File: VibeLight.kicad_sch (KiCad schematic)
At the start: 7 parts, among them SW1 SW_Push, SW2 SW_Push, U1 OPT3002-ALS, U2 ADXL343

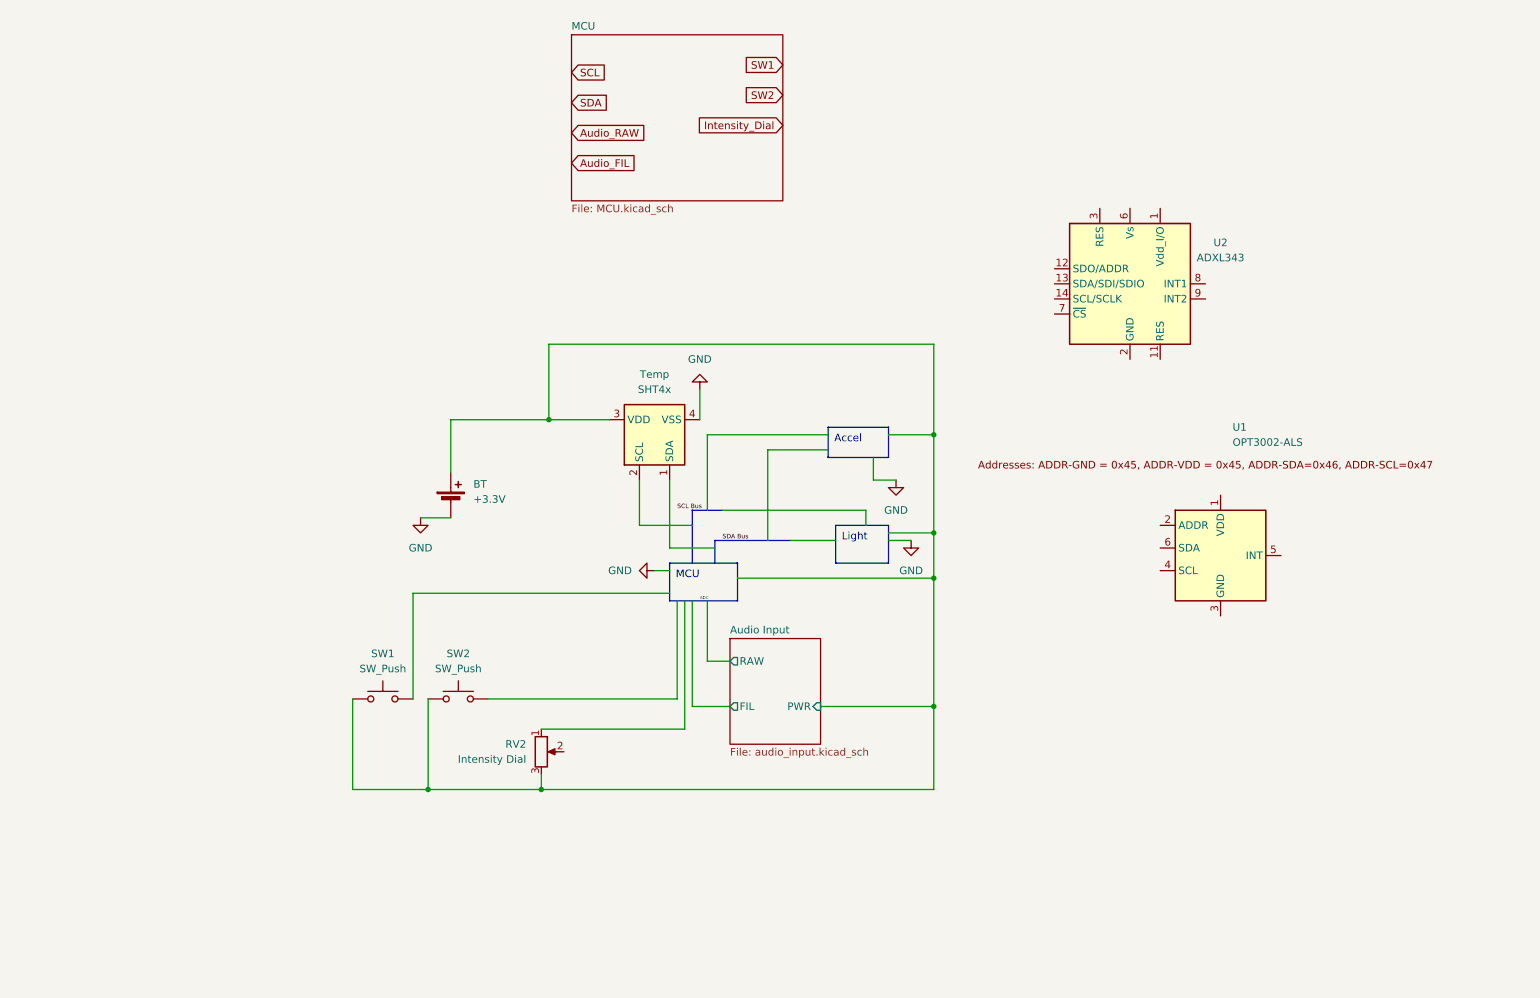
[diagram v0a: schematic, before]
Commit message: misc changes during call
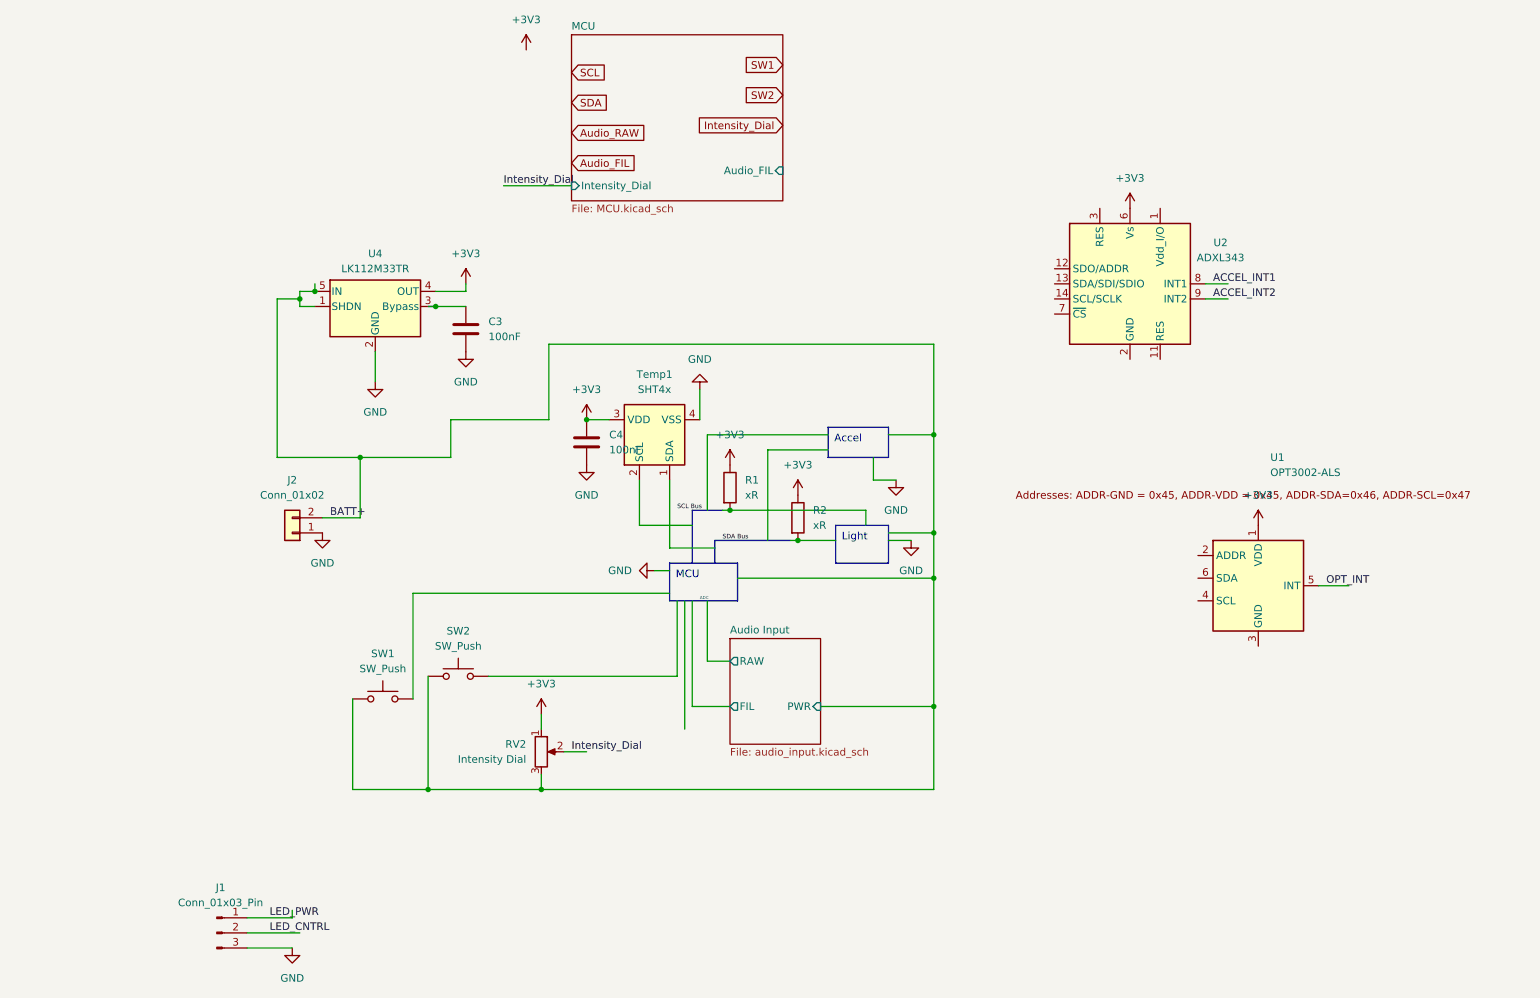
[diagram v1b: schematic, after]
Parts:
- removed BT: +3.3V, symbol Device:Battery_Cell
- added C3, C4: 100nF, Capacitor_SMD:C_0603_1608Metric_Pad1.08x0.95mm_HandSolder, symbol Device:C
- added J1: Conn_01x03_Pin, symbol Connector:Conn_01x03_Pin
- added J2: Conn_01x02, symbol Connector_Generic:Conn_01x02
- added R1, R2: xR, Resistor_SMD:R_0603_1608Metric_Pad0.98x0.95mm_HandSolder, symbol Device:R
- added U4: LK112M33TR, Package_TO_SOT_SMD:SOT-23-5, symbol Regulator_Linear:LK112M33TR
- RV2: footprint Potentiometer_SMD:Potentiometer_ACP_CA6-VSMD_Vertical -> Potentiometer_SMD:Potentiometer_Bourns_TC33X_Vertical; Source (none) -> https://www.digikey.com/en/products/detail/bourns-inc/TC33X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
- SW1, SW2: footprint (none) -> Button_Switch_SMD:SW_Push_1P1T_NO_CK_KMR2; Source (none) -> https://www.digikey.com/en/products/detail/c-k-va/KMR223GLF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
- renumbered Temp to Temp1
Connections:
- net GND: now also C3.2, C4.2, J1.3 (Pin_3), J2.1 (Pin_1), U4.2 (GND)
- net Intensity_Dial: now also RV2.2
- net +3V3: now reaches RV2.1
- net +3V3: now also Temp1.3 (VDD), U1.1 (VDD), U2.6 (Vs), C4.1, R1.1, R2.1, U4.4 (OUT)
- net ACCEL_INT1: now reaches U2.8 (INT1)
- net ACCEL_INT2: now reaches U2.9 (INT2)
- net OPT_INT: now reaches U1.5 (INT)
- net Audio Input/PWR renamed BATT+
- net BATT+: now also J2.2 (Pin_2), U4.1 (SHDN), U4.5 (IN); no longer Temp1.3 (VDD)
- new net: C3.1, U4.3 (Bypass)
- new net LED_CNTRL: J1.2 (Pin_2)
- new net LED_PWR: J1.1 (Pin_1)
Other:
- sheet MCU ports: added Audio_FIL, Intensity_Dial; removed none
- moved on the sheet: SW2, U1

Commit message: started work on pcb layout
started work on pcb layout
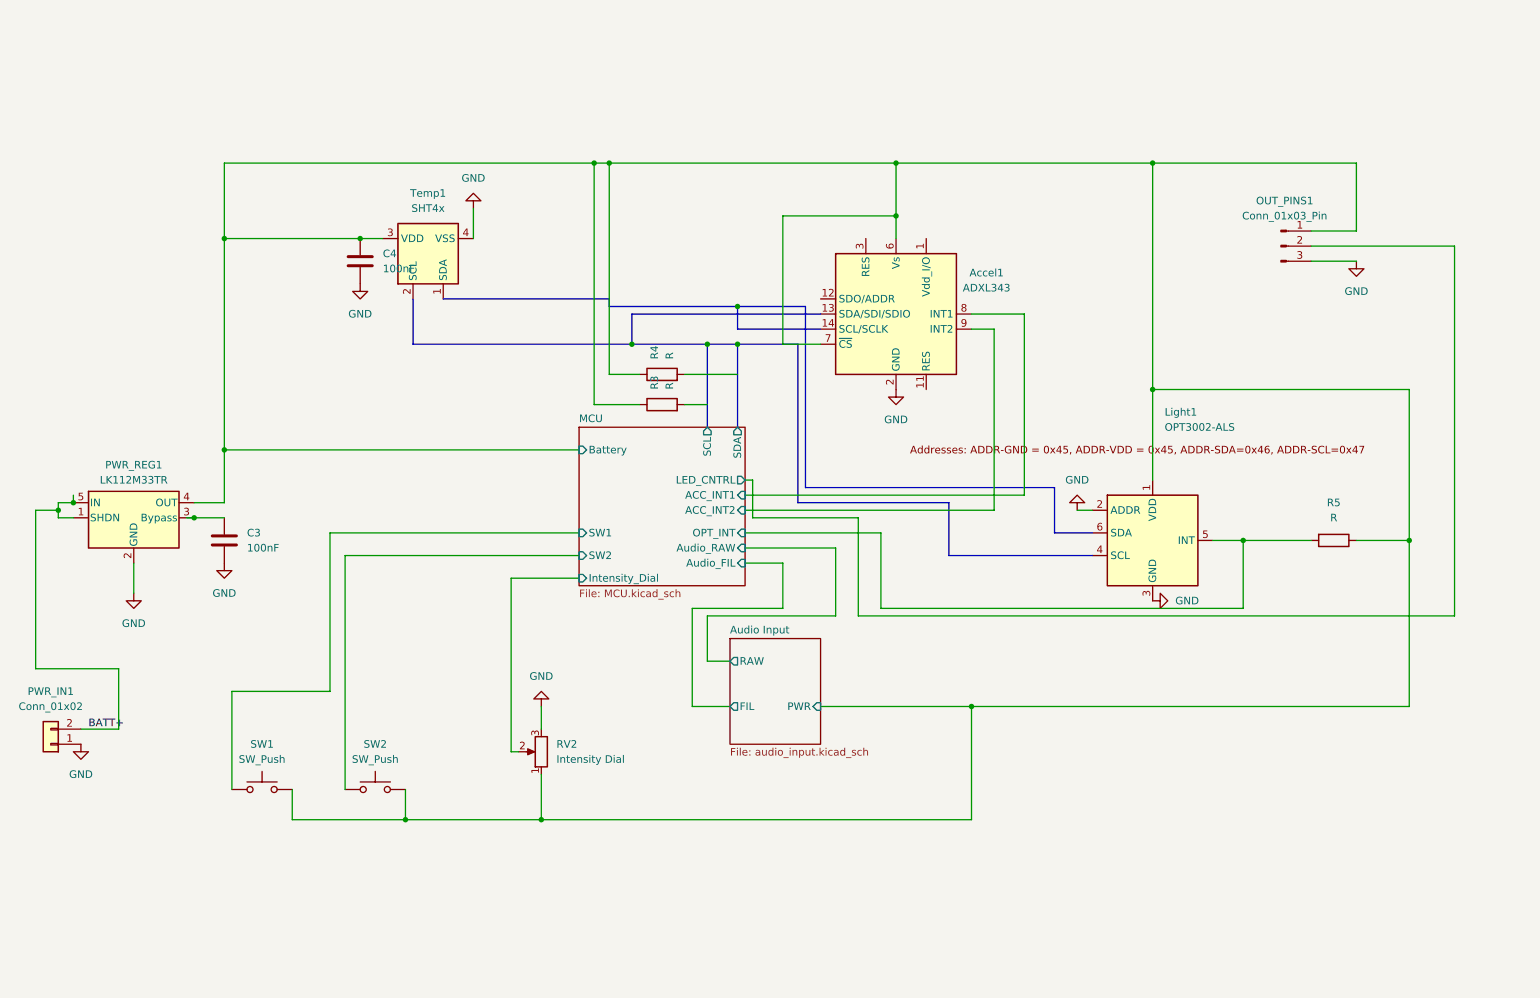
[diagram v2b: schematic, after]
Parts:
- removed R1, R2: xR, Resistor_SMD:R_0603_1608Metric_Pad0.98x0.95mm_HandSolder, symbol Device:R
- added R3, R4, R5: R, Resistor_SMD:R_0603_1608Metric_Pad0.98x0.95mm_HandSolder, symbol Device:R
- renumbered U2 to Accel1, U1 to Light1, J1 to OUT_PINS1, J2 to PWR_IN1, U4 to PWR_REG1
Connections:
- net +3V3 is gone; now on net Audio Input/PWR: Accel1.6 (Vs), C4.1, Light1.1 (VDD), PWR_REG1.4 (OUT), RV2.1, Temp1.3 (VDD)
- net LED_PWR is gone; now on net Audio Input/PWR: OUT_PINS1.1 (Pin_1)
- net BATT+: no longer RV2.3, SW1.1, SW2.1
- net GND: now also Accel1.2 (GND), Accel1.4 (GND), Accel1.5 (GND), Light1.2 (NC), Light1.3 (GND), RV2.3
- net Audio Input/PWR: now reaches SW2.2
- net Audio Input/PWR: now also Accel1.7 (~{CS}), SW1.2, R3.1, R4.1, R5.1
- net ACCEL_INT1 renamed MCU/ACC_INT1
- net ACCEL_INT2 renamed MCU/ACC_INT2
- net Intensity_Dial renamed MCU/Intensity_Dial
- net LED_CNTRL renamed MCU/LED_CNTRL
- net OPT_INT renamed MCU/OPT_INT
- net MCU/OPT_INT: now also R5.2
- new net MCU/SW1: SW1.1
- new net MCU/SW2: SW2.1
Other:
- sheet MCU ports: added ACC_INT1, ACC_INT2, Audio_RAW, Battery, LED_CNTRL, OPT_INT, SCL, SDA, SW1, SW2; removed none
- note removed: "ADC"
- moved on the sheet: Accel1, C3, C4, Light1, OUT_PINS1, PWR_IN1, PWR_REG1, RV2, SW1, SW2, Temp1
